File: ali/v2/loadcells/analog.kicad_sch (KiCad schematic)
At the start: 16 parts, among them J9 Conn_01x04, U5 ADS1261

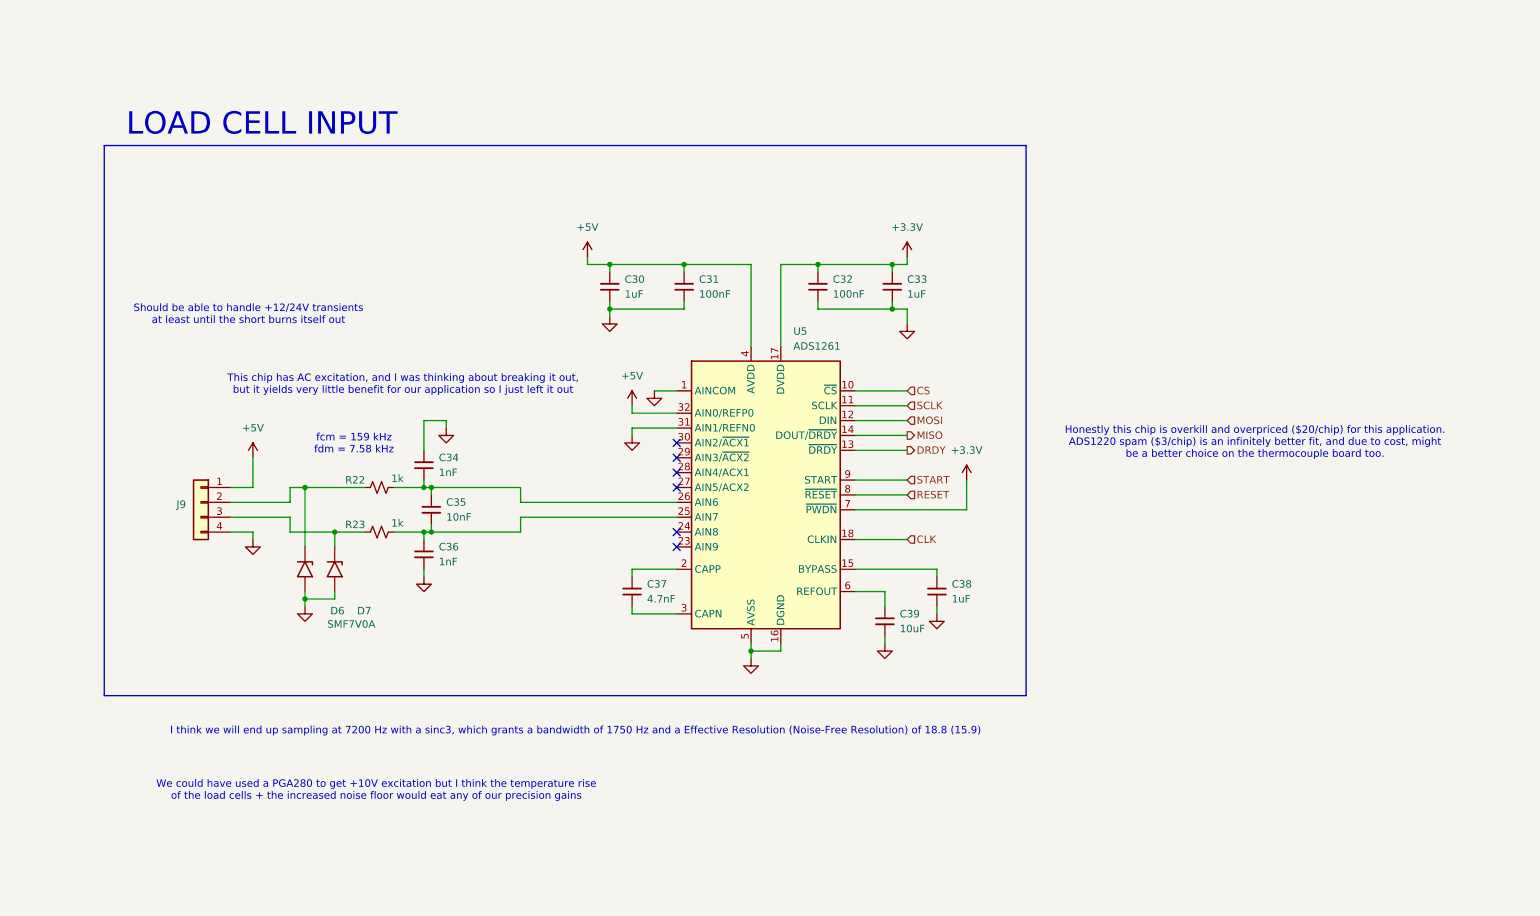
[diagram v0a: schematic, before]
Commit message: Begin prep for second board review
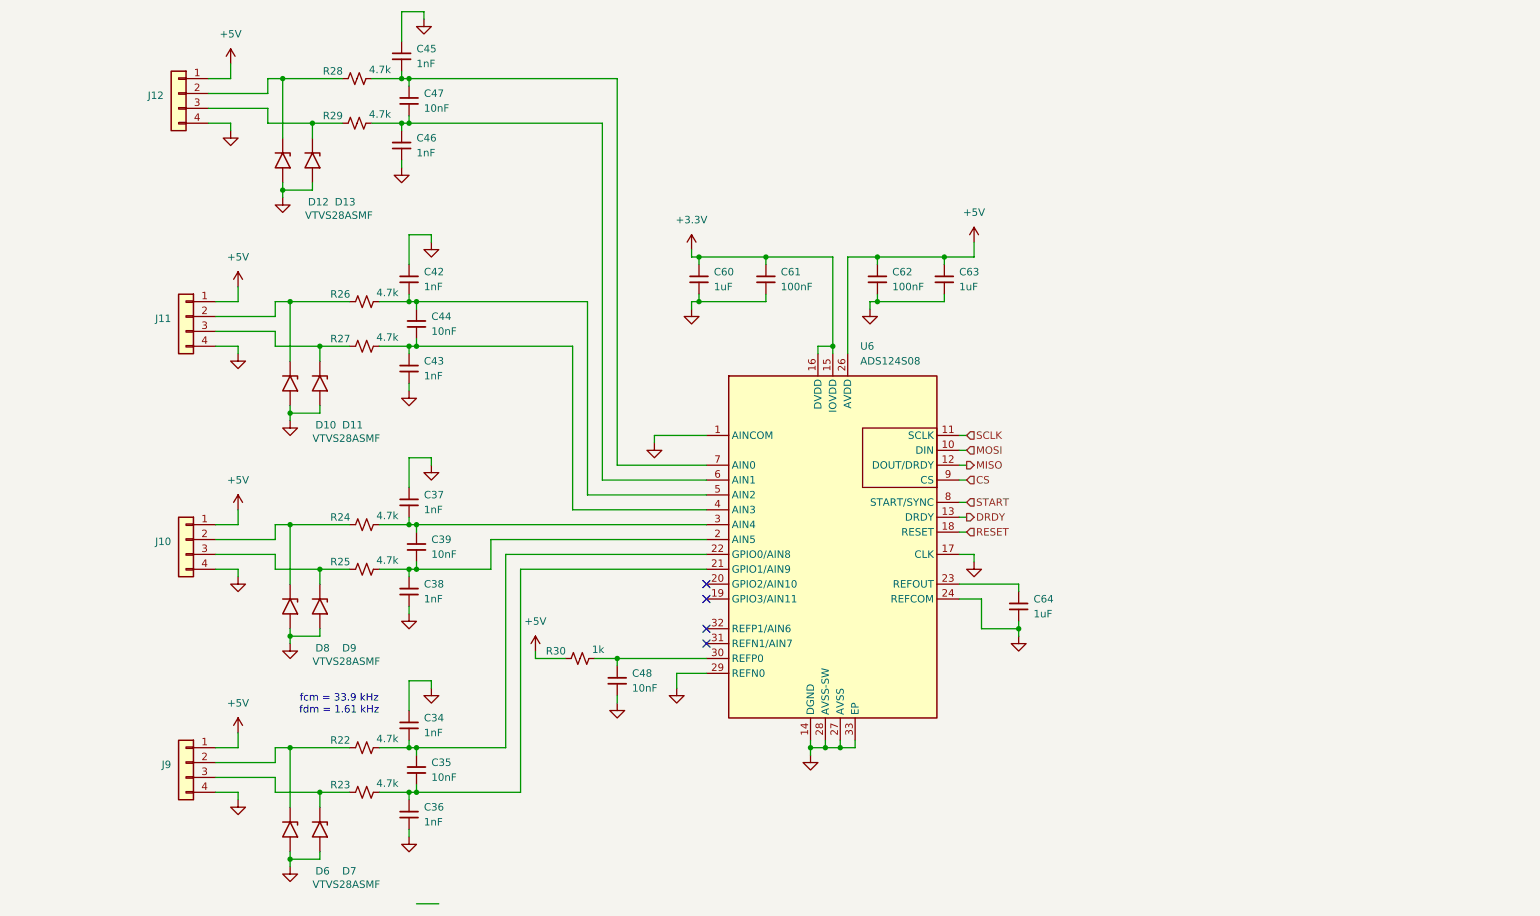
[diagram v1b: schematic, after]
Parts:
- removed C30, C33: 1uF, APRL_Passive:C_0603, symbol Device:C_Small
- removed C31, C32: 100nF, APRL_Passive:C_0603, symbol Device:C_Small
- removed U5: ADS1261, APRL_Package_QFN:Texas_RHB0032E_VQFN-32-1EP_5x5mm_P0.5mm_EP3.45x3.45mm_ThermalVias, symbol APRL_Analog:ADS1261
- added C42, C43, C45, C46: 1nF, APRL_Passive:C_0603, symbol Device:C_Small
- added C44, C47, C48: 10nF, APRL_Passive:C_0603, symbol Device:C_Small
- added C60, C63, C64: 1uF, APRL_Passive:C_0603, symbol Device:C_Small
- added C61, C62: 100nF, APRL_Passive:C_0603, symbol Device:C_Small
- added D10, D11, D12, D13, D8, D9: VTVS28ASMF, Diode_SMD:D_SMF, symbol Diode:SMF5V0A
- added J10, J11, J12: Conn_01x04, APRL_Connector_Molex:Molex_CLIK-Mate_503159-0401_1x04-1MP_P1.50mm_Vertical, symbol Connector_Generic:Conn_01x04
- added R24, R25, R26, R27, R28, R29: 4.7k, APRL_Passive:R_0603, symbol Device:R_Small_US
- added R30: 1k, APRL_Passive:R_0603, symbol Device:R_Small_US
- added U6: ADS124S08, APRL_Package_QFN:Texas_RHB0032M_VQFN-32-1EP_5x5mm_P0.5mm_EP2.1x2.1mm_ThermalVias, symbol APRL_Analog:ADS124S08
- C37: value 4.7nF -> 1nF; MPN GRM1885C1H472JA01 -> GRM1885C1H102FA01
- C38: value 1uF -> 1nF; MPN GRM188D72A105KE01 -> GRM1885C1H102FA01
- C39: value 10uF -> 10nF; MPN GRM188R61A106KE69 -> GRM1885C1H103JA01
- D6, D7: value SMF7V0A -> VTVS28ASMF; MPN SMF7V0A-E3-18 -> VTVS28ASMF-M3-08
- R22, R23: value 1k -> 4.7k; MPN RT0603BRD071KL -> RT0603BRD074K7L
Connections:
- net +3.3V: now also C60.1, C61.1, U6.15 (IOVDD), U6.16 (DVDD)
- net +5V: now also C62.1, C63.1, J10.1 (Pin_1), J11.1 (Pin_1), J12.1 (Pin_1), R30.1, U6.26 (AVDD)
- net CS: now also U6.9 (CS)
- net DRDY: now also U6.13 (DRDY)
- net GND: now also C37.2, C38.1, C42.2, C43.1, C45.2, C46.1, C48.1, C60.2, C61.2, C62.2, C63.2, C64.2, D10.2 (A2), D11.2 (A2), D12.2 (A2), D13.2 (A2), D8.2 (A2), D9.2 (A2), J10.4 (Pin_4), J11.4 (Pin_4), J12.4 (Pin_4), U6.1 (AINCOM), U6.14 (DGND), U6.17 (CLK), U6.24 (REFCOM), U6.27 (AVSS), U6.28 (AVSS-SW), U6.29 (REFN0), U6.33 (EP); no longer C38.2, C39.2
- net MISO: now also U6.12 (DOUT/DRDY)
- net MOSI: now also U6.10 (DIN)
- net RESET: now also U6.18 (RESET)
- net SCLK: now also U6.11 (SCLK)
- net START: now also U6.8 (START/SYNC)
- net at C35.1, C36.2, R23.2: now also U6.21 (GPIO1/AIN9)
- net at C34.1, C35.2, R22.2: now also U6.22 (GPIO0/AIN8)
- net at C39.1: now also C38.2, R25.2, U6.2 (AIN5)
- net at C37.1: now also C39.2, R24.2, U6.3 (AIN4)
- new net: D10.1 (A1), J11.2 (Pin_2), R26.1
- new net: D11.1 (A1), J11.3 (Pin_3), R27.1
- new net: D12.1 (A1), J12.2 (Pin_2), R28.1
- new net: C45.1, C47.2, R28.2, U6.7 (AIN0)
- new net: D9.1 (A1), J10.3 (Pin_3), R25.1
- new net: D13.1 (A1), J12.3 (Pin_3), R29.1
- new net: C43.2, C44.1, R27.2, U6.4 (AIN3)
- new net: D8.1 (A1), J10.2 (Pin_2), R24.1
- new net: C46.2, C47.1, R29.2, U6.6 (AIN1)
- new net: C42.1, C44.2, R26.2, U6.5 (AIN2)
- new net: C64.1, U6.23 (REFOUT)
- new net: C48.2, R30.2, U6.30 (REFP0)
- no-connect marks 6 -> 4
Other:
- note added: "fcm = 33.9 kHz fdm = 1.61 kHz"
- note removed: "Honestly this chip is overkill and overpriced ($20/chip) for this application. ADS1220 spam ($3/chip) is an infinitely better fit, and due to cost, might be a better choice on the thermocouple board too."
- note removed: "I think we will end up sampling at 7200 Hz with a sinc3, which grants a bandwidth of 1750 Hz and a Effective Resolution (Noise-Free Resolution) of 18.8 (15.9)"
- note removed: "LOAD CELL INPUT"
- note removed: "Should be able to handle +12/24V transients at least until the short burns itself out"
- note removed: "This chip has AC excitation, and I was thinking about breaking it out, but it yields very little benefit for our application so I just left it out"
- note removed: "We could have used a PGA280 to get +10V excitation but I think the temperature rise of the load cells + the increased noise floor would eat any of our precision gains"
- note removed: "fcm = 159 kHz fdm = 7.58 kHz"
